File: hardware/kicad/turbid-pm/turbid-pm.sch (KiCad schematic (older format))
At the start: 10 parts, among them J1 Raspbery Pi, J2 PMS 7003, J3 Turbidity sensor

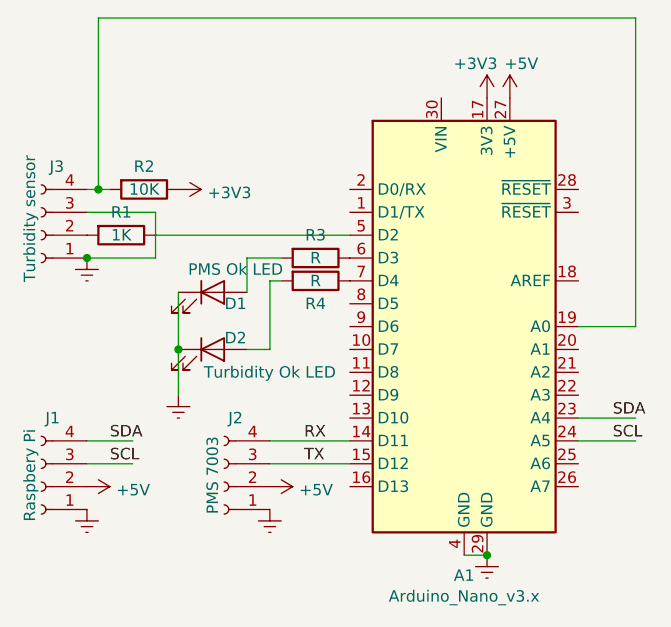
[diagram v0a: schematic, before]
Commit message: added 3d print source
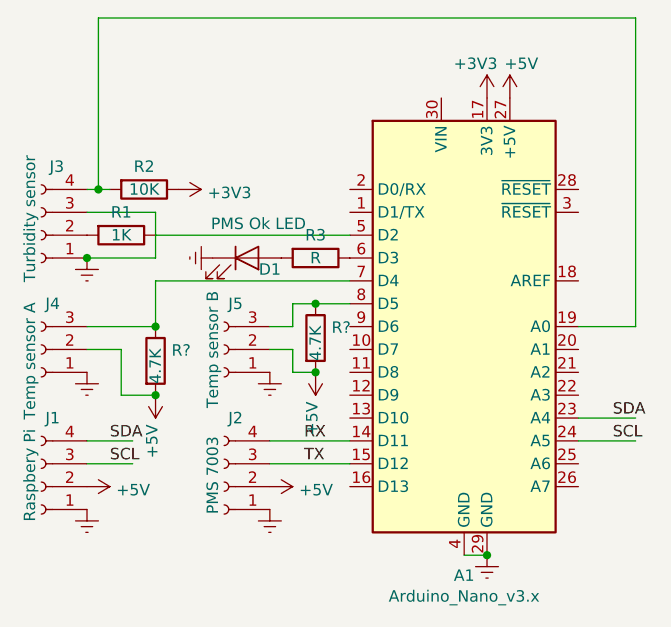
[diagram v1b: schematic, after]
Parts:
- removed D2: Turbidity Ok LED, LED_THT:LED_D3.0mm_Clear, symbol Device:LED
- removed R4: R, Resistor_THT:R_Axial_DIN0207_L6.3mm_D2.5mm_P10.16mm_Horizontal, symbol Device:R
- added J4: Temp sensor A, Connector_PinSocket_2.54mm:PinSocket_1x03_P2.54mm_Vertical, symbol Connector:Conn_01x03_Female
- added J5: Temp sensor B, Connector_PinSocket_2.54mm:PinSocket_1x03_P2.54mm_Vertical, symbol Connector:Conn_01x03_Female
- added R? (x2): 4.7K, symbol Device:R
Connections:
- wire segments 24 -> 30
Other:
- moved on the sheet: D1
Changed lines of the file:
@@
 L Device:LED D1
 U 1 1 5EA6A9A5
-P 4200 3100
-F 0 "D1" H 4300 3050 50  0000 C CNN
-F 1 "PMS Ok LED" H 4300 3200 50  0000 C CNN
-F 2 "LED_THT:LED_D3.0mm_Clear" H 4200 3100 50  0001 C CNN
-F 3 "~" H 4200 3100 50  0001 C CNN
-	1    4200 3100
-	1    0    0    -1
-$EndComp
-$Comp
-L Device:LED D2
-U 1 1 5EA6B3A9
-P 4200 3350
-F 0 "D2" H 4300 3400 50  0000 C CNN
-F 1 "Turbidity Ok LED" H 4450 3250 50  0000 C CNN
-F 2 "LED_THT:LED_D3.0mm_Clear" H 4200 3350 50  0001 C CNN
-F 3 "~" H 4200 3350 50  0001 C CNN
-	1    4200 3350
+P 4350 2950
+F 0 "D1" H 4450 2900 50  0000 C CNN
+F 1 "PMS Ok LED" H 4400 3100 50  0000 C CNN
+F 2 "LED_THT:LED_D3.0mm_Clear" H 4350 2950 50  0001 C CNN
+F 3 "~" H 4350 2950 50  0001 C CNN
+	1    4350 2950
 	1    0    0    -1
 $EndComp
@@
 $EndComp
 $Comp
-L Device:R R4
-U 1 1 5EA6C26A
-P 4650 3050
-F 0 "R4" V 4750 3050 50  0000 C CNN
-F 1 "R" V 4650 3050 50  0000 C CNN
-F 2 "Resistor_THT:R_Axial_DIN0207_L6.3mm_D2.5mm_P10.16mm_Horizontal" V 4580 3050 50  0001 C CNN
-F 3 "~" H 4650 3050 50  0001 C CNN
-	1    4650 3050
+L power:Earth #PWR0111
+U 1 1 5EA764BF
+P 4200 2950
+F 0 "#PWR0111" H 4200 2700 50  0001 C CNN
+F 1 "Earth" H 4200 2800 50  0001 C CNN
+F 2 "" H 4200 2950 50  0001 C CNN
+F 3 "~" H 4200 2950 50  0001 C CNN
+	1    4200 2950
 	0    1    1    0
 $EndComp
-$Comp
-L power:Earth #PWR0111
-U 1 1 5EA764BF
-P 4050 3550
-F 0 "#PWR0111" H 4050 3300 50  0001 C CNN
-F 1 "Earth" H 4050 3400 50  0001 C CNN
-F 2 "" H 4050 3550 50  0001 C CNN
-F 3 "~" H 4050 3550 50  0001 C CNN
-	1    4050 3550
-	1    0    0    -1
-$EndComp
-Wire Wire Line
-	4350 3100 4350 2950
-Wire Wire Line
-	4350 2950 4500 2950
-Wire Wire Line
-	4500 3050 4450 3050
-Wire Wire Line
-	4450 3050 4450 3350
-Wire Wire Line
-	4450 3350 4350 3350
-Wire Wire Line
-	4050 3100 4050 3350
-Connection ~ 4050 3350
-Wire Wire Line
-	4050 3350 4050 3550
 Wire Wire Line
 	3650 2750 3950 2750
@@
 Wire Wire Line
 	3950 2750 3950 2950
+$Comp
+L Connector:Conn_01x03_Female J4
+U 1 1 5EAA80C9
+P 3450 3350
+F 0 "J4" H 3400 3150 50  0000 C CNN
+F 1 "Temp sensor A" V 3500 3400 50  0000 C CNN
+F 2 "Connector_PinSocket_2.54mm:PinSocket_1x03_P2.54mm_Vertical" H 3450 3350 50  0001 C CNN
+F 3 "~" H 3450 3350 50  0001 C CNN
+	1    3450 3350
+	-1   0    0    1
+$EndComp
+$Comp
+L power:+5V #PWR0110
+U 1 1 5EAA9807
+P 3950 3550
+F 0 "#PWR0110" H 3950 3400 50  0001 C CNN
+F 1 "+5V" V 3965 3678 50  0000 L CNN
+F 2 "" H 3950 3550 50  0001 C CNN
+F 3 "" H 3950 3550 50  0001 C CNN
+	1    3950 3550
+	-1   0    0    1
+$EndComp
+Wire Wire Line
+	3950 3050 3950 3250
+Wire Wire Line
+	3950 3250 3650 3250
+$Comp
+L power:Earth #PWR0112
+U 1 1 5EABE03A
+P 3650 3450
+F 0 "#PWR0112" H 3650 3200 50  0001 C CNN
+F 1 "Earth" H 3650 3300 50  0001 C CNN
+F 2 "" H 3650 3450 50  0001 C CNN
+F 3 "~" H 3650 3450 50  0001 C CNN
+	1    3650 3450
+	1    0    0    -1
+$EndComp
+$Comp
+L Connector:Conn_01x03_Female J5
+U 1 1 5EAC2BEB
+P 4250 3350
+F 0 "J5" H 4200 3150 50  0000 C CNN
+F 1 "Temp sensor B" V 4300 3350 50  0000 C CNN
+F 2 "Connector_PinSocket_2.54mm:PinSocket_1x03_P2.54mm_Vertical" H 4250 3350 50  0001 C CNN
+F 3 "~" H 4250 3350 50  0001 C CNN
+	1    4250 3350
+	-1   0    0    1
+$EndComp
+$Comp
+L power:+5V #PWR0113
+U 1 1 5EAC2BF5
+P 4650 3450
+F 0 "#PWR0113" H 4650 3300 50  0001 C CNN
+F 1 "+5V" V 4665 3578 50  0000 L CNN
+F 2 "" H 4650 3450 50  0001 C CNN
+F 3 "" H 4650 3450 50  0001 C CNN
+	1    4650 3450
+	-1   0    0    1
+$EndComp
+$Comp
+L power:Earth #PWR0114
+U 1 1 5EAC2C01
+P 4450 3450
+F 0 "#PWR0114" H 4450 3200 50  0001 C CNN
+F 1 "Earth" H 4450 3300 50  0001 C CNN
+F 2 "" H 4450 3450 50  0001 C CNN
+F 3 "~" H 4450 3450 50  0001 C CNN
+	1    4450 3450
+	1    0    0    -1
+$EndComp
+Wire Wire Line
+	3950 3050 4800 3050
+Wire Wire Line
+	4800 3150 4650 3150
+$Comp
+L Device:R R?
+U 1 1 5EAD302D
+P 3950 3400
+F 0 "R?" H 4020 3446 50  0000 L CNN
+F 1 "4.7K" V 3950 3300 50  0000 L CNN
+F 2 "" V 3880 3400 50  0001 C CNN
+F 3 "~" H 3950 3400 50  0001 C CNN
+	1    3950 3400
+	1    0    0    -1
+$EndComp
+Connection ~ 3950 3250
+$Comp
+L Device:R R?
+U 1 1 5EAD38D1
+P 4650 3300
+F 0 "R?" H 4720 3346 50  0000 L CNN
+F 1 "4.7K" V 4650 3200 50  0000 L CNN
+F 2 "" V 4580 3300 50  0001 C CNN
+F 3 "~" H 4650 3300 50  0001 C CNN
+	1    4650 3300
+	1    0    0    -1
+$EndComp
+Connection ~ 4650 3150
+Wire Wire Line
+	4450 3350 4550 3350
+Wire Wire Line
+	4550 3350 4550 3450
+Wire Wire Line
+	4550 3450 4650 3450
+Connection ~ 4650 3450
+Wire Wire Line
+	3650 3350 3800 3350
+Wire Wire Line
+	3800 3350 3800 3550
+Wire Wire Line
+	3800 3550 3950 3550
+Connection ~ 3950 3550
+Wire Wire Line
+	4450 3250 4550 3250
+Wire Wire Line
+	4550 3250 4550 3150
+Wire Wire Line
+	4550 3150 4650 3150
 $EndSCHEMATC
